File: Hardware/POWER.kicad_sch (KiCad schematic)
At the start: 65 parts, among them J201 5V_USB, J202 Battery IN, U202 AP2112K-3.3, U203 AP2112K-1.8, U204 AP2112K-3.3

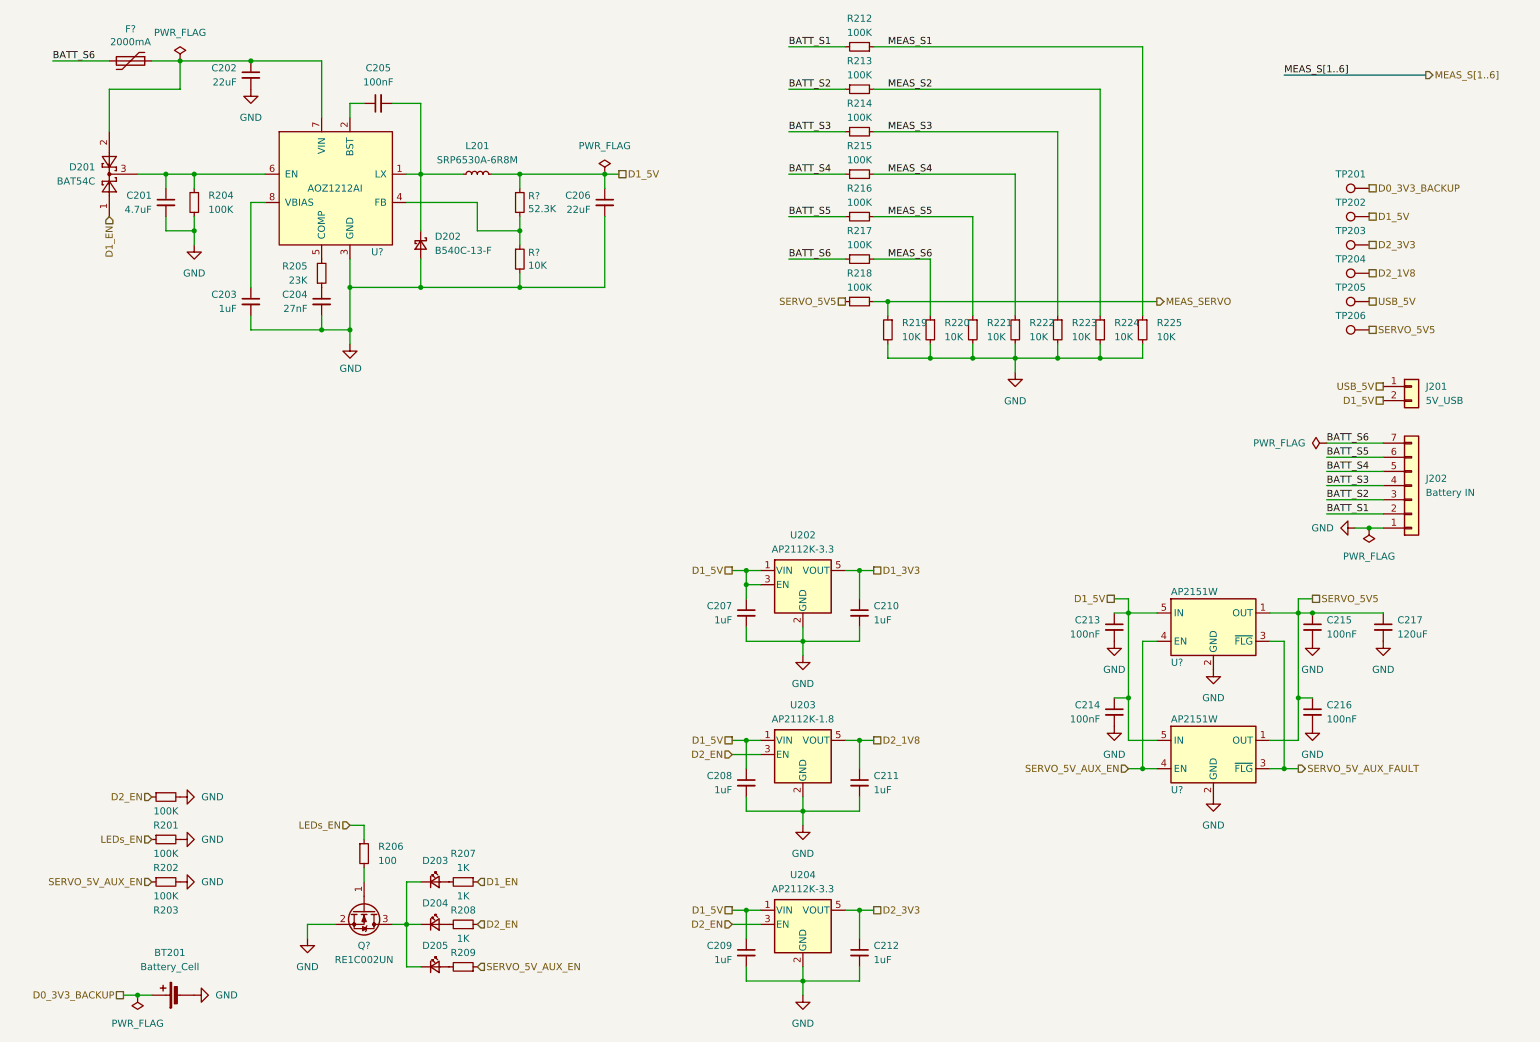
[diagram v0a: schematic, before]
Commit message: Checkpoint
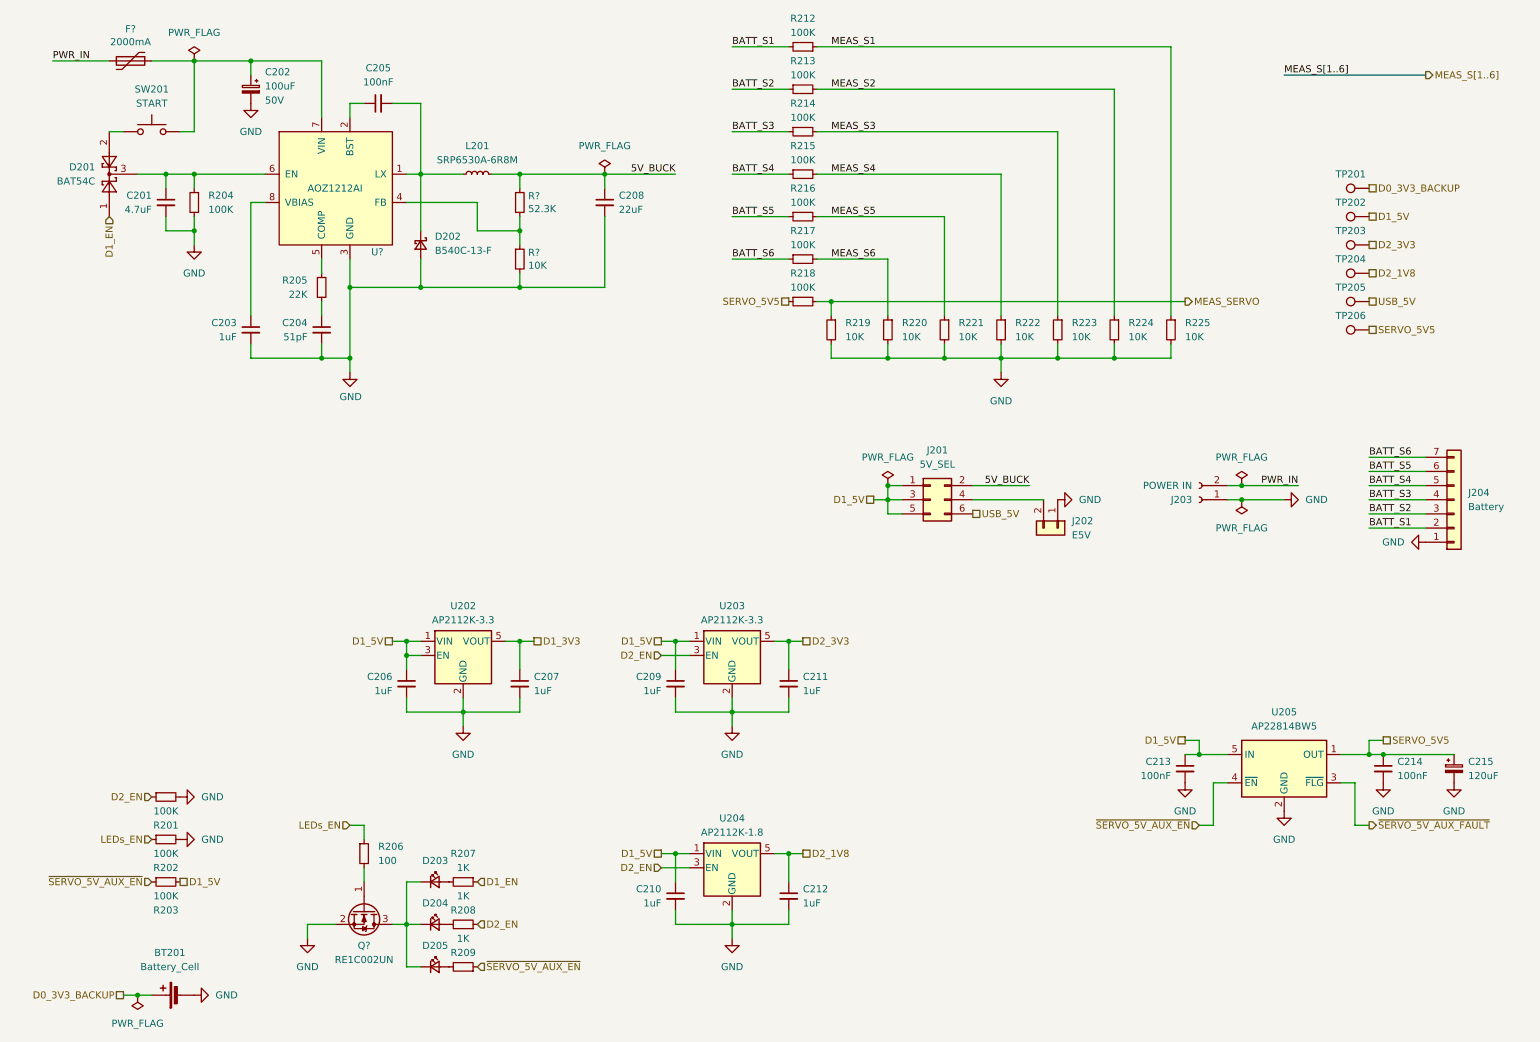
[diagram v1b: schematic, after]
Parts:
- removed C214, C216: 100nF, symbol Device:C_Small
- removed U? (x2): AP2151W, Package_TO_SOT_SMD:SOT-23-5, symbol leptunKicadLib:AP2151W
- added J201: 5V_SEL, Connector_PinHeader_2.54mm:PinHeader_2x03_P2.54mm_Vertical, symbol Connector_Generic:Conn_02x03_Odd_Even
- added J203: POWER IN, symbol Connector:Conn_01x02_Socket
- added SW201: START, symbol Switch:SW_Push
- added U205: AP22814BW5, Package_TO_SOT_SMD:SOT-23-5, symbol Power_Management:AP22814BW5
- C201: footprint (none) -> Capacitor_SMD:C_1206_3216Metric
- C202: value 22uF -> 100uF; footprint (none) -> Capacitor_THT:C_Radial_D8.0mm_H11.5mm_P3.50mm; symbol Device:C_Small -> Device:C_Polarized_Small; Rating (none) -> 50V
- C203, C209: footprint (none) -> Capacitor_SMD:C_0805_2012Metric
- C204: value 27nF -> 51pF; footprint (none) -> Capacitor_SMD:C_0402_1005Metric
- C205, C213: footprint (none) -> Capacitor_SMD:C_0603_1608Metric
- C206: renamed from C207; footprint (none) -> Capacitor_SMD:C_0805_2012Metric
- C207: renamed from C210; footprint (none) -> Capacitor_SMD:C_0805_2012Metric
- C208: renamed from C206; footprint (none) -> Capacitor_SMD:C_1210_3225Metric
- C210: renamed from C208; footprint (none) -> Capacitor_SMD:C_0805_2012Metric
- C211: renamed from C212; footprint (none) -> Capacitor_SMD:C_0805_2012Metric
- C212: renamed from C211; footprint (none) -> Capacitor_SMD:C_0805_2012Metric
- C214: renamed from C215; footprint (none) -> Capacitor_SMD:C_0603_1608Metric
- C215: renamed from C217; symbol Device:C_Small -> Device:C_Polarized_Small
- J202: renamed from J201; value 5V_USB -> E5V
- J204: renamed from J202; value Battery IN -> Battery
- R201, R202, R203, R204, R206, R207, R208, R209, R212, R213, R214, R215, R216, R217, R218: footprint (none) -> Resistor_SMD:R_0805_2012Metric
- R205: value 23K -> 22K; footprint (none) -> Resistor_SMD:R_0805_2012Metric
- R219, R220, R221, R222, R223, R224, R225, R? (x2): footprint (none) -> Resistor_SMD:R_0603_1608Metric
- renumbered U204 to U203, U203 to U204
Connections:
- net BATT_S6: no longer F?.2
- net D1_5V: now also R203.2, J201.1 (Pin_1), J201.3 (Pin_3), J201.5 (Pin_5), U205.5 (IN); no longer C208.1, J202.2 (Pin_2), L201.2, R?.1
- net GND: now also J202.1 (Pin_1), J203.1 (Pin_1), U205.2 (GND); no longer R203.2
- net SERVO_5V5: now also U205.1 (OUT)
- net USB_5V: now also J201.6 (Pin_6); no longer J202.1 (Pin_1)
- net at C202.1, F?.1, U?.7 (VIN): now also SW201.2; no longer D201.2
- net SERVO_5V_AUX_EN renamed ~{SERVO_5V_AUX_EN}
- net ~{SERVO_5V_AUX_EN}: now also U205.4 (~{EN})
- new net: J201.4 (Pin_4), J202.2 (Pin_2)
- new net: D201.2, SW201.1
- new net 5V_BUCK: C208.1, J201.2 (Pin_2), L201.2, R?.1
- new net PWR_IN: F?.2, J203.2 (Pin_2)
- new net ~{SERVO_5V_AUX_FAULT}: U205.3 (~{FLG})
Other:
- moved on the sheet: C203, C204, C206, C207, C209, C210, C211, C212, C213, C214, J202, J204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

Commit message: Checkpoint
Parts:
- F?: footprint Fuse:Fuse_1206_3216Metric -> (none)
- J203: footprint (none) -> Connector_AMASS:AMASS_XT30UPB-M_1x02_P5.0mm_Vertical
- J204: footprint (none) -> Connector_PinHeader_2.54mm:PinHeader_1x07_P2.54mm_Vertical
- TP201, TP202, TP203, TP204, TP205, TP206: footprint (none) -> TestPoint:TestPoint_Pad_D2.0mm
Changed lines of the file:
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@@
       (effects (font (size 1.27 1.27)) (justify left))
     )
-    (property "Footprint" "" (at 226.06 101.6 0)
+    (property "Footprint" "Connector_AMASS:AMASS_XT30UPB-M_1x02_P5.0mm_Vertical" (at 226.06 101.6 0)
       (effects (font (size 1.27 1.27)) hide)
     )
@@
       (effects (font (size 1.27 1.27)) hide)
     )
-    (property "Footprint" "" (at 256.54 45.72 0)
+    (property "Footprint" "TestPoint:TestPoint_Pad_D2.0mm" (at 256.54 45.72 0)
       (effects (font (size 1.27 1.27)) hide)
     )
@@
       (effects (font (size 1.27 1.27)) hide)
     )
-    (property "Footprint" "" (at 256.54 50.8 0)
+    (property "Footprint" "TestPoint:TestPoint_Pad_D2.0mm" (at 256.54 50.8 0)
       (effects (font (size 1.27 1.27)) hide)
     )
@@
       (effects (font (size 1.27 1.27)) hide)
     )
-    (property "Footprint" "" (at 256.54 40.64 0)
+    (property "Footprint" "TestPoint:TestPoint_Pad_D2.0mm" (at 256.54 40.64 0)
       (effects (font (size 1.27 1.27)) hide)
     )
@@
       (effects (font (size 1.27 1.27)) hide)
     )
-    (property "Footprint" "" (at 256.54 55.88 0)
+    (property "Footprint" "TestPoint:TestPoint_Pad_D2.0mm" (at 256.54 55.88 0)
       (effects (font (size 1.27 1.27)) hide)
     )
@@
       (effects (font (size 1.27 1.27)) hide)
     )
-    (property "Footprint" "" (at 256.54 66.04 0)
+    (property "Footprint" "TestPoint:TestPoint_Pad_D2.0mm" (at 256.54 66.04 0)
       (effects (font (size 1.27 1.27)) hide)
     )
@@
       (effects (font (size 1.27 1.27)) (justify left))
     )
-    (property "Footprint" "" (at 271.78 101.6 0)
+    (property "Footprint" "Connector_PinHeader_2.54mm:PinHeader_1x07_P2.54mm_Vertical" (at 271.78 101.6 0)
       (effects (font (size 1.27 1.27)) hide)
     )
@@
       (effects (font (size 1.27 1.27)))
     )
-    (property "Footprint" "Fuse:Fuse_1206_3216Metric" (at 29.21 24.13 0)
+    (property "Footprint" "" (at 29.21 24.13 0)
       (effects (font (size 1.27 1.27)) (justify left) hide)
     )
@@
       (effects (font (size 1.27 1.27)) hide)
     )
-    (property "Footprint" "" (at 256.54 60.96 0)
-      (effects (font (size 1.27 1.27)) hide)
-    )
+    (property "Footprint" "TestPoint:TestPoint_Pad_D2.0mm" (at 256.54 60.96 0)
+      (effects (font (size 1.27 1.27)) hide)
+    )

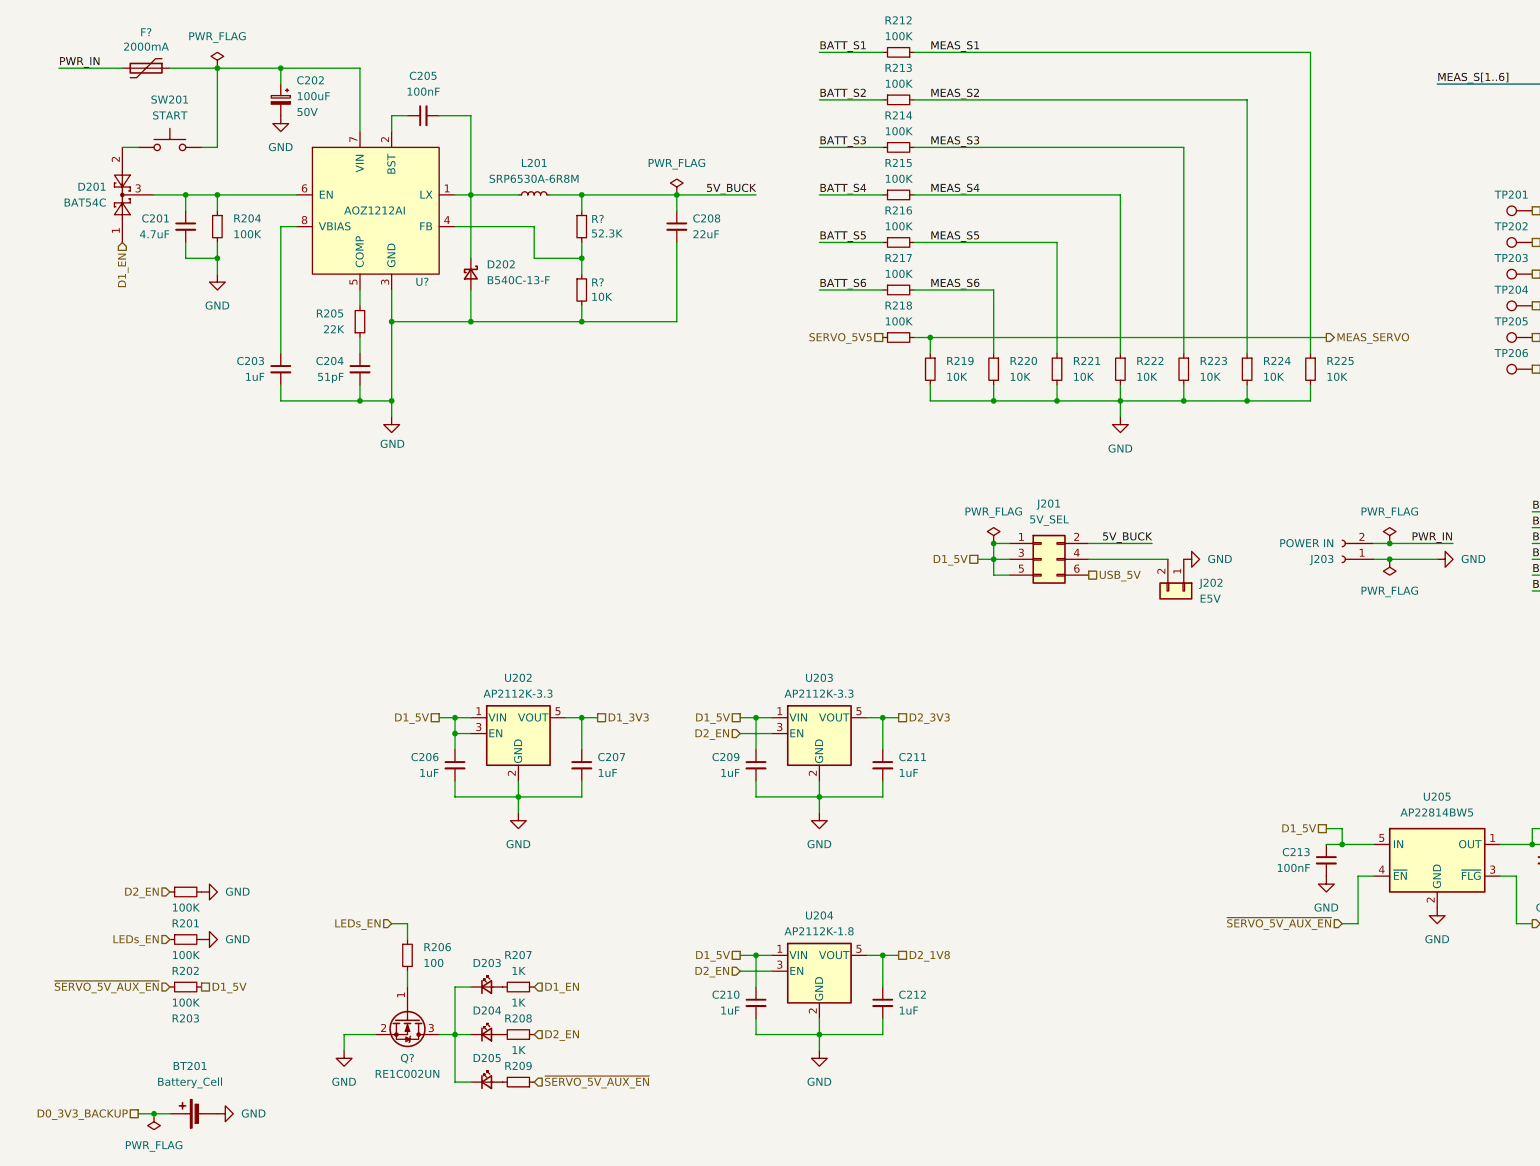
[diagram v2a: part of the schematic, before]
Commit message: Checkpoint
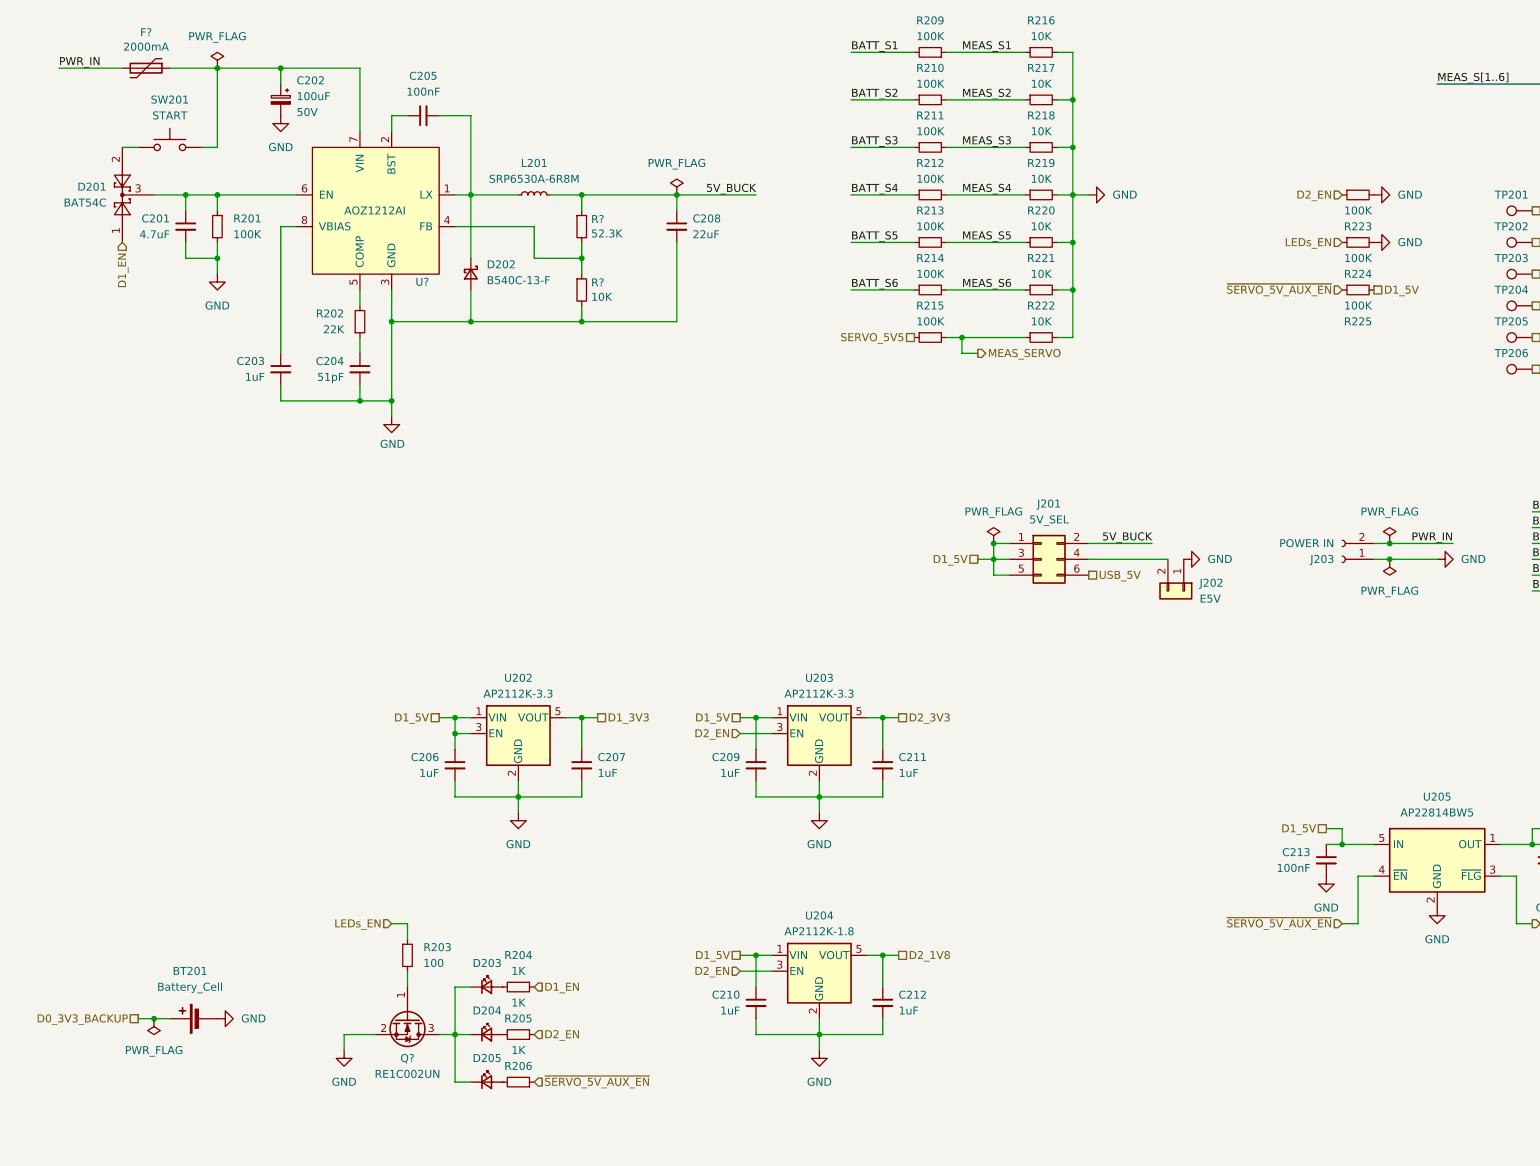
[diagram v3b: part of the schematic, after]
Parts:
- D203, D204, D205: footprint (none) -> LED_SMD:LED_1206_3216Metric
- F?: footprint (none) -> Fuse:Fuse_1812_4532Metric
- SW201: footprint (none) -> Button_Switch_THT:SW_PUSH_6mm_H5mm
- renumbered R204 to R201, R205 to R202, R206 to R203, R207 to R204, R208 to R205, R209 to R206, R212 to R209, R213 to R210, R214 to R211, R215 to R212, R216 to R213, R217 to R214, R218 to R215, R225 to R216, R224 to R217, R223 to R218, R222 to R219, R221 to R220, R220 to R221, R219 to R222, R201 to R223, R202 to R224, R203 to R225
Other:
- moved on the sheet: BT201, R209, R210, R211, R212, R213, R214, R215, R216, R217, R218, R219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

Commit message: Checkpoint
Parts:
- added C201, C203, C211, C217: 1uF, Capacitor_SMD:C_0805_2012Metric, symbol Device:C_Small
- added C204, C212: 100nF, Capacitor_SMD:C_0603_1608Metric, symbol Device:C_Small
- added C214: 22uF, Capacitor_SMD:C_1210_3225Metric, symbol Device:C_Small
- added D206, D207, D208: ~, LED_SMD:LED_1206_3216Metric, symbol Device:LED_Small
- added R202, R203, R208, R216: 100K, Resistor_SMD:R_0805_2012Metric, symbol Device:R_Small
- added R224: 10K, Resistor_SMD:R_0603_1608Metric, symbol Device:R_Small
- added R231, R232, R233: 1K, Resistor_SMD:R_0805_2012Metric, symbol Device:R_Small
- added TP201, TP202: ~, TestPoint:TestPoint_Pad_D2.0mm, symbol Connector:TestPoint
- added U201, U206: AP2112K-3.3, Package_TO_SOT_SMD:SOT-23-5, symbol Regulator_Linear:AP2112K-3.3
- added U203: AP2151W, Package_TO_SOT_SMD:SOT-23-5, symbol leptunKicadLib:AP2151W
- renumbered C201 to C202, C202 to C205, C203 to C206, C204 to C207, C205 to C208, C206 to C213, C211 to C215, C212 to C216, C207 to C218, C208 to C219, C213 to C220, C214 to C221, C215 to C222, J204 to J201, J203 to J202, J201 to J203, J202 to J204, R202 to R204, R223 to R207, R225 to R209, R209 to R210, R210 to R211, R211 to R212, R212 to R213, R213 to R214, R214 to R215, R215 to R217, R216 to R218, R217 to R219, R218 to R220, R219 to R221, R220 to R222, R221 to R223, R222 to R225, R203 to R226, R224 to R227, R204 to R228, R205 to R229, R206 to R230, TP201 to TP204, TP202 to TP205, TP204 to TP206, TP206 to TP207, TP205 to TP208, U203 to U204, U204 to U205, U202 to U207, U205 to U208
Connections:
- net D1_3V3: now also TP206.1
- net D1_5V: now also R228.1, TP208.1, C201.1, C204.1, C211.1, R216.1, U201.1 (VIN), U203.5 (IN), U206.1 (VIN); no longer TP205.1
- net D1_EN: no longer R228.1
- net D2_1V8: now also TP204.1; no longer TP206.1
- net D2_3V3: now also R229.1
- net D2_EN: no longer R229.1
- net GND: now also C201.2, C203.2, C204.2, C211.2, C212.2, C214.2, C217.2, R202.1, R203.2, R208.2, R224.2, U201.2 (GND), U203.2 (GND), U206.2 (GND)
- net SERVO_5V5: now also R233.1
- net USB_5V: no longer TP208.1
- net ~{SERVO_5V_AUX_EN}: no longer R230.1
- net at D203.1 (K), D204.1 (K), D205.1 (K)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: now also D206.1 (K), D207.1 (K), D208.1 (K)
- net D0_3V3_BACKUP renamed D0_VBAT
- net D0_VBAT: no longer TP204.1
- new net: D207.2 (A), R232.2
- new net: D208.2 (A), R233.2
- new net: D206.2 (A), R231.2
- new net D3_3V3: C203.1, R230.1, TP201.1, U201.5 (VOUT)
- new net D3_EN: R203.1, U201.3 (EN)
- new net D4_3V3: C217.1, R231.1, TP205.1, U206.5 (VOUT)
- new net D4_EN: R208.1, U206.3 (EN)
- new net D5_5V: C212.1, C214.1, R232.1, TP202.1, U203.1 (OUT)
- new net D5_EN: R202.2, U203.4 (EN)
- new net MEAS_D1_5V: R216.2, R224.1
- new net ~{D5_FAULT}: U203.3 (~{FLG})
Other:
- moved on the sheet: BT201, C202, C205, C206, C207, C208, C209, C210, C213, C215, C216, C218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
